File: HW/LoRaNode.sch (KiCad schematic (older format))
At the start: 3 parts

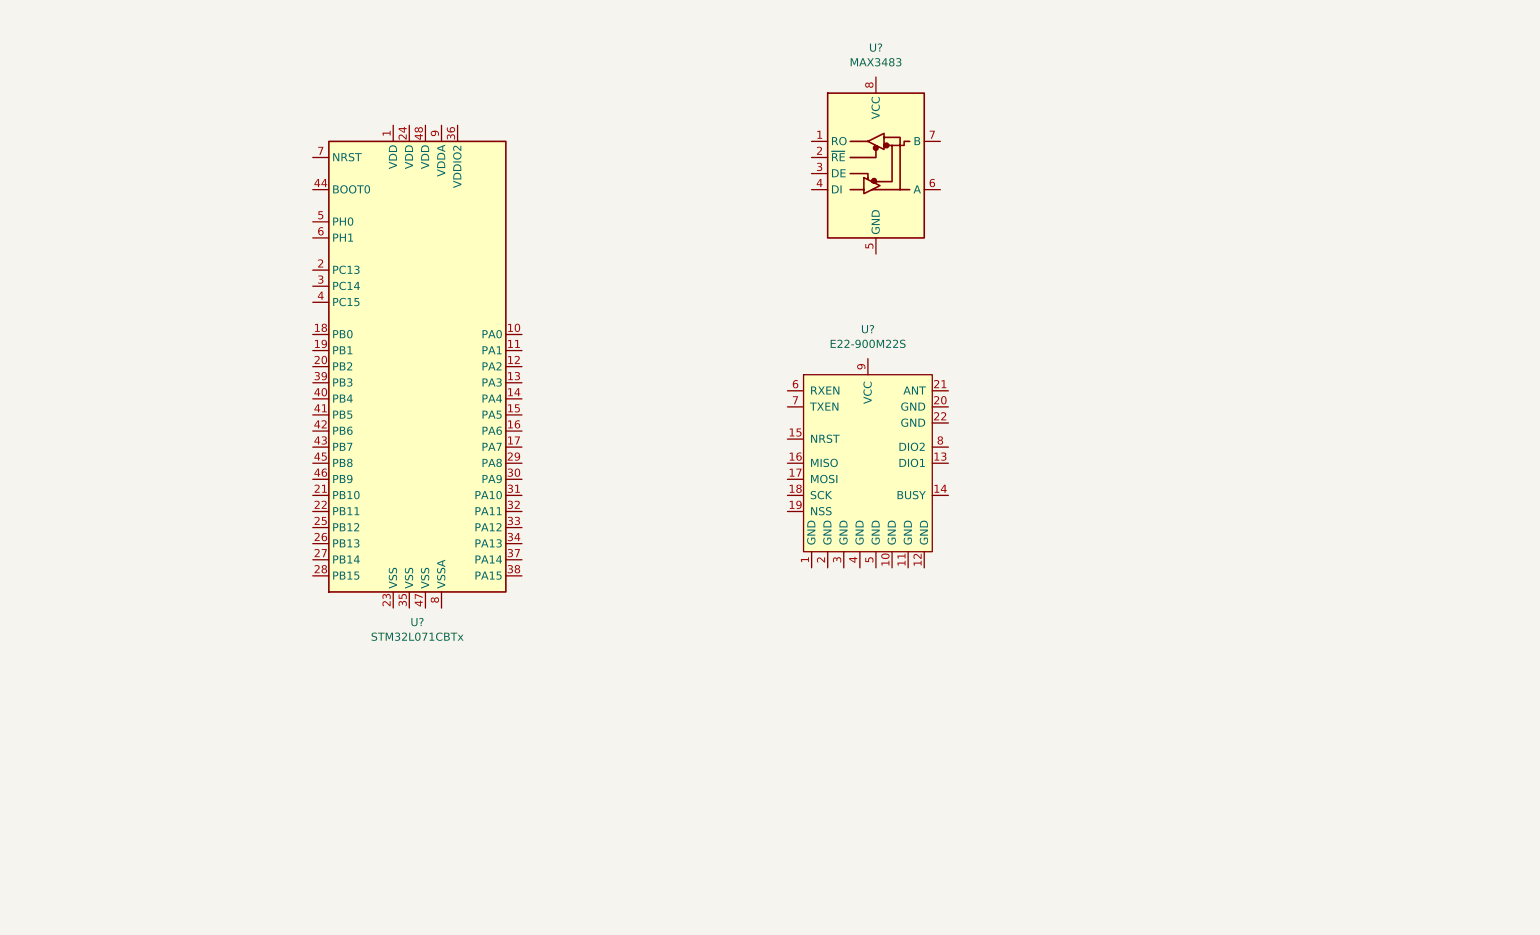
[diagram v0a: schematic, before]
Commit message: update some schematic design
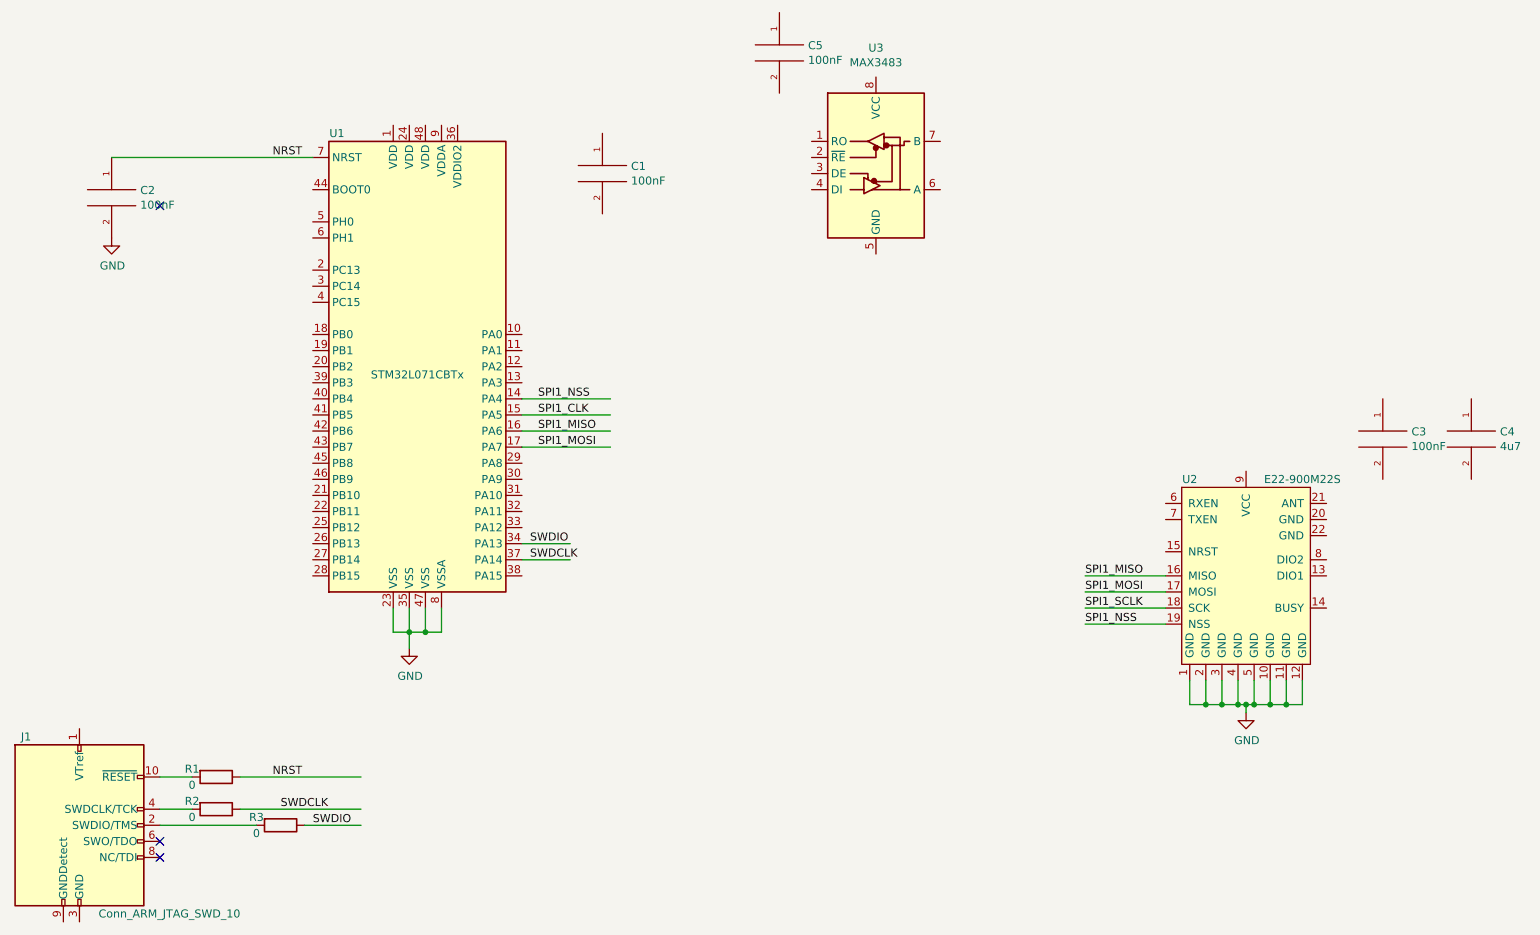
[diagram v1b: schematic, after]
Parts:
- added C1, C2, C3, C5: 100nF, Capacitor_SMD:C_0402_1005Metric, symbol pspice:CAP
- added C4: 4u7, Capacitor_SMD:C_0603_1608Metric, symbol pspice:CAP
- added J1: Conn_ARM_JTAG_SWD_10, Connector_PinHeader_1.27mm:PinHeader_2x05_P1.27mm_Vertical_SMD, symbol Connector:Conn_ARM_JTAG_SWD_10
- added R1, R2, R3: 0, Resistor_SMD:R_0402_1005Metric, symbol Device:R
- U3: renamed from U?; footprint (none) -> Package_SO:SO-8_3.9x4.9mm_P1.27mm
- gave numbers to parts that had none: 2
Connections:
- net labels added: GND, NRST, SPI1_CLK, SPI1_MISO, SPI1_MOSI, SPI1_NSS, SPI1_SCLK, SWDCLK, SWDIO
- wire segments 0 -> 42
- no-connect marks 0 -> 3
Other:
- moved on the sheet: U2
